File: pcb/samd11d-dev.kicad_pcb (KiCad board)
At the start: 2 copper layers, 30.5 x 29.2 mm, 28 parts, among them J1 Conn_02x05_Odd_Even, J2 USB_B_Micro, J3 Conn_01x08, J4 Conn_01x08, SW1 SW_Push, SW2 SW_Push, U1 ATSAMD11D14A-SS, U3 MCP1700-3302E_SOT23, U4 USBLC6-2SC6, Y1 32.768 kHz

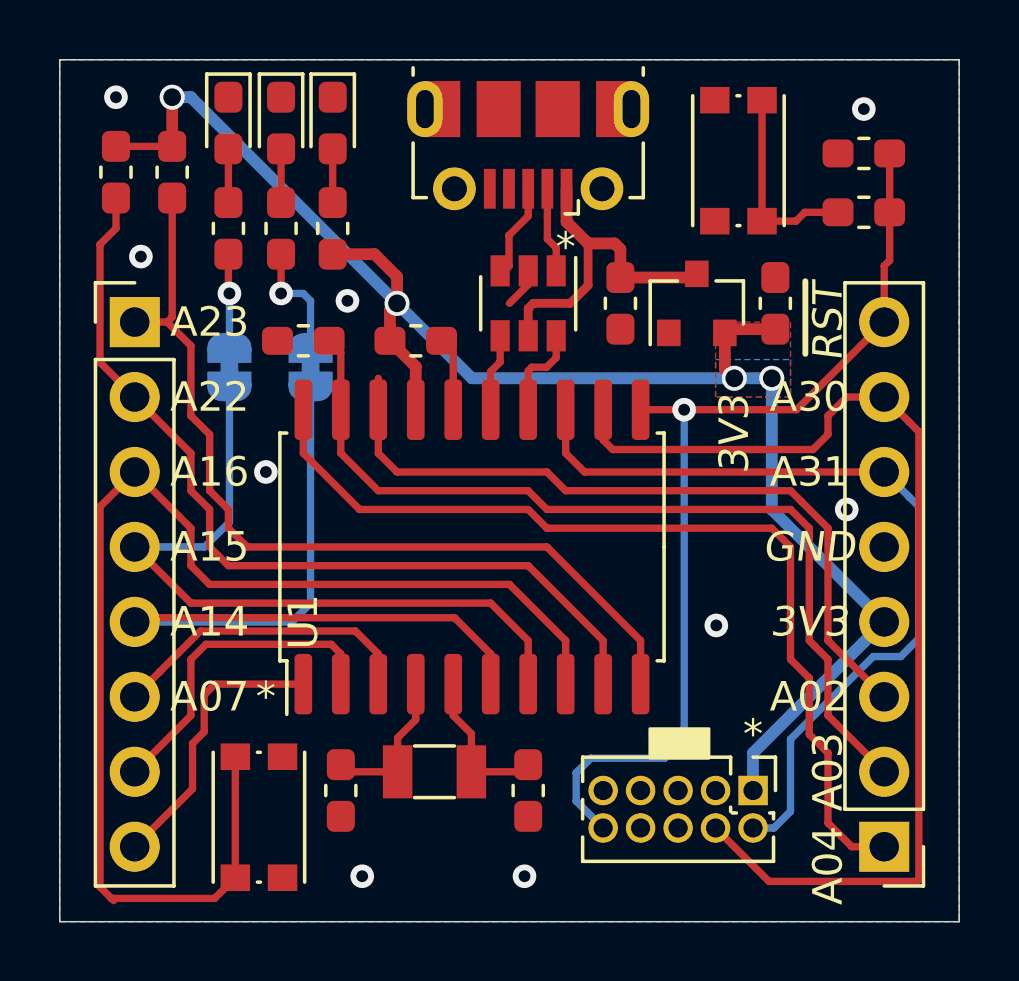
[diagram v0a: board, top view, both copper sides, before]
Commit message: Complete new layout for v0.21
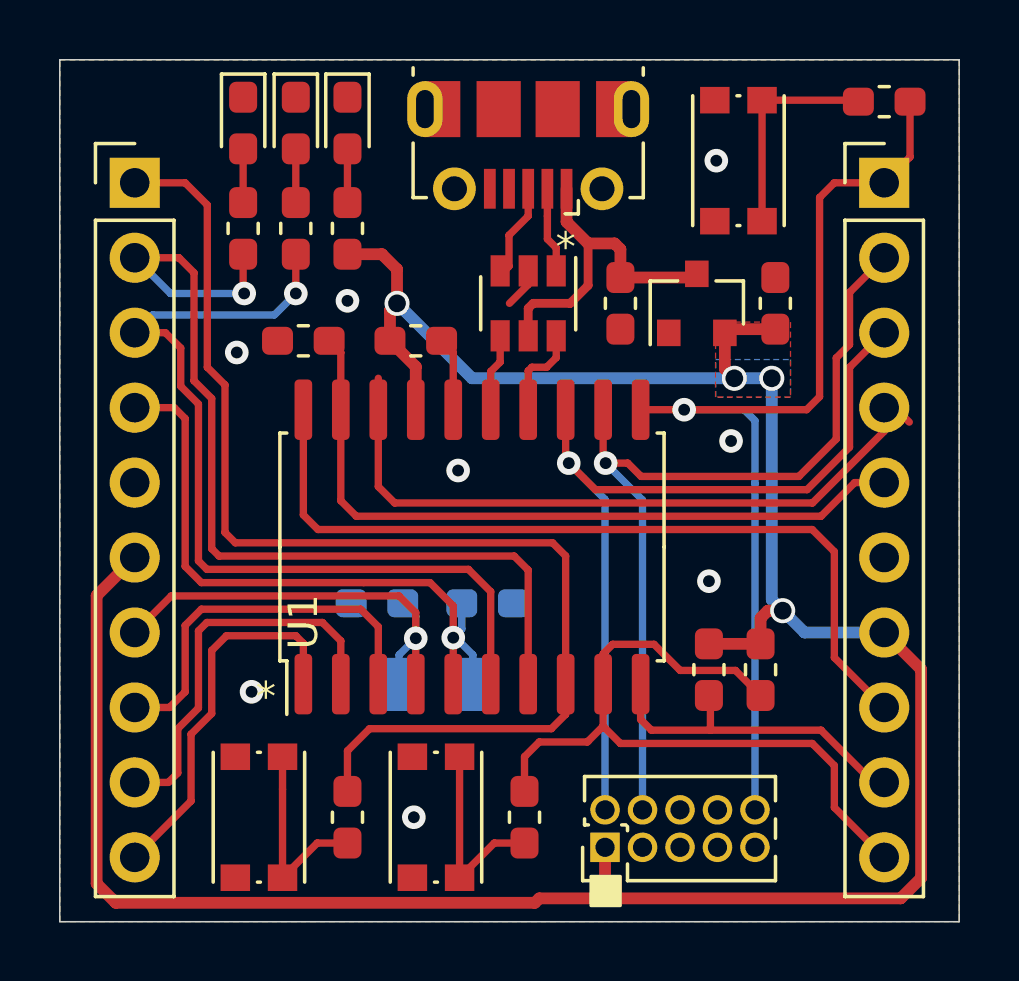
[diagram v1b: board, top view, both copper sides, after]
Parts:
- removed C7: 100n, Capacitor_SMD:C_0603_1608Metric_Pad1.05x0.95mm_HandSolder
- removed JP1, JP2: Jumper_NC_Small, Jumper:SolderJumper-2_P1.3mm_Bridged_RoundedPad1.0x1.5mm
- added R7: 330R, Resistor_SMD:R_0603_1608Metric_Pad1.05x0.95mm_HandSolder, F.Cu at (134.8, 126.5)
- added R8: 330R, Resistor_SMD:R_0603_1608Metric_Pad1.05x0.95mm_HandSolder, F.Cu at (140.8, 126.5)
- added SW3: SW_Push, Button_Switch_SMD:SW_Push_1P1T_NO_CK_KMR2, F.Cu at (137.8, 126.5)
- C1, C2, Y1: moved to B.Cu
- J3, J4: value Conn_01x08 -> Conn_01x10; footprint Connector_PinHeader_2.54mm:PinHeader_1x08_P2.54mm_Vertical -> Connector_PinHeader_2.54mm:PinHeader_1x10_P2.54mm_Vertical
- moved R1 27.6 mm to (148.8, 121.5)
- moved R2 24.8 mm to (147.0, 121.5)
- moved J4 22.5 mm to (152.9, 105.0), turned to 0 degrees
- moved C2 6.49 mm to (139.5, 119.2), turned to 0 degrees
- moved C1 6.46 mm to (135.8, 119.2), turned to 180 degrees
- moved J1 5.37 mm to (143.5, 127.5), turned to 90 degrees
- moved J3 4.72 mm to (127.5, 105.0)
- moved R6 3.81 mm to (152.9, 102.2)
- moved Y1 2.96 mm to (137.8, 122.0)
- moved D1 0.50 mm to (131.2, 103.0)
- moved D2 0.50 mm to (133.0, 103.0)
- moved D3 0.50 mm to (134.8, 103.0)
- moved R3 0.50 mm to (131.2, 106.5)
- moved R4 0.50 mm to (134.8, 106.5)
- moved R5 0.50 mm to (133.0, 106.5)
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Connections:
- C1 pad 1: Net-(C1-Pad1) -> /PA08
- C2 pad 1: Net-(C2-Pad1) -> /PA09
- J3 pad 1: /PA23 -> /PA16
- J3 pad 2: /PA22 -> /PA15
- J3 pad 3: /PA16 -> /PA14
- J3 pad 4: /PA15 -> /PA09
- J3 pad 5: /PA14 -> GND
- J3 pad 6: /PA07 -> +3V3
- J3 pad 7: /PA06 -> /PA08
- J3 pad 8: /PA05 -> /PA07
- J4 pad 1: /PA04 -> /~RST
- J4 pad 2: /PA03 -> /PA30
- J4 pad 3: /PA02 -> /PA31
- J4 pad 4: +3V3 -> /PA02
- J4 pad 5: GND -> /PA03
- J4 pad 6: /PA31 -> GND
- J4 pad 7: /PA30 -> +3V3
- J4 pad 8: /~RST -> /PA04
- R3 pad 1: Net-(JP2-Pad2) -> /PA15
- R5 pad 1: Net-(JP1-Pad2) -> /PA14
- SW2 pad 1: /PA16 -> Net-(R7-Pad1)
- U1 pad 4: Net-(C1-Pad1) -> /PA08
- U1 pad 5: Net-(C2-Pad1) -> /PA09
- Y1 pad 1: Net-(C1-Pad1) -> /PA08
- Y1 pad 2: Net-(C2-Pad1) -> /PA09
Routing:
- net +3V3: track 56.0 -> 90.2 mm
- net /PA09: track 0.00 -> 22.4 mm, vias 0 -> 1
- net /PA23: track 30.2 -> 11.5 mm
- net /PA08: track 0.00 -> 15.9 mm, vias 0 -> 1
- net /PA15: track 24.3 -> 32.3 mm, vias 0 -> 1
- net Net-(R7-Pad1): track 0.00 -> 6.85 mm
- net Net-(R8-Pad1): track 0.00 -> 6.79 mm
- net /PA30: track 36.3 -> 29.7 mm, vias 0 -> 1
- net /PA03: track 30.2 -> 24.7 mm
- net Net-(C2-Pad1): track 5.25 -> 0.00 mm
- net Net-(C1-Pad1): track 5.25 -> 0.00 mm
- net /PA22: track 29.7 -> 25.1 mm
- net Net-(JP1-Pad2): track 4.03 -> 0.00 mm, vias 1 -> 0
- net /PA04: track 31.4 -> 28.1 mm
- net /PA05: track 9.63 -> 12.9 mm
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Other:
- board text added: "A08"
- board text added: "A09"
- board text removed: "SAMD11D-dev v0.2"
- board text removed: "awjlogan 2020"

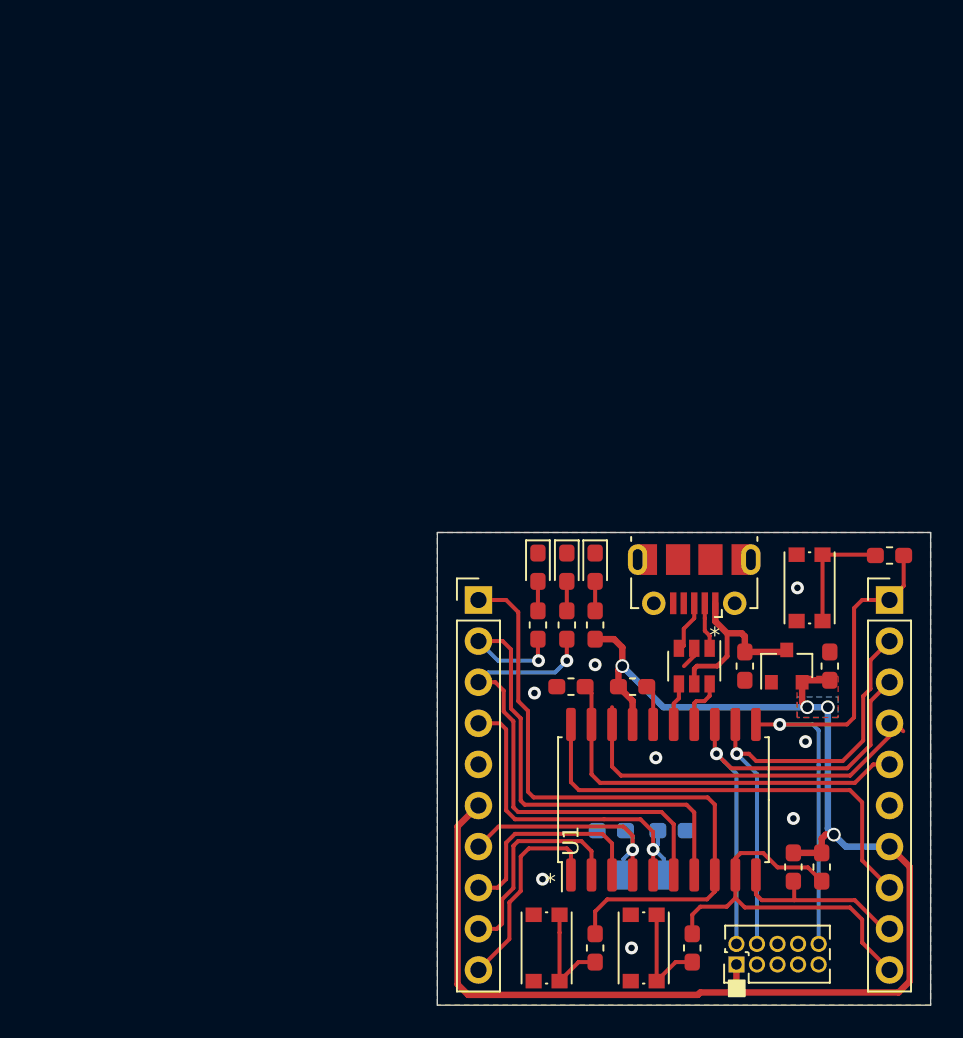
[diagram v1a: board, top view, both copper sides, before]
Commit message: v2.1 manufactured
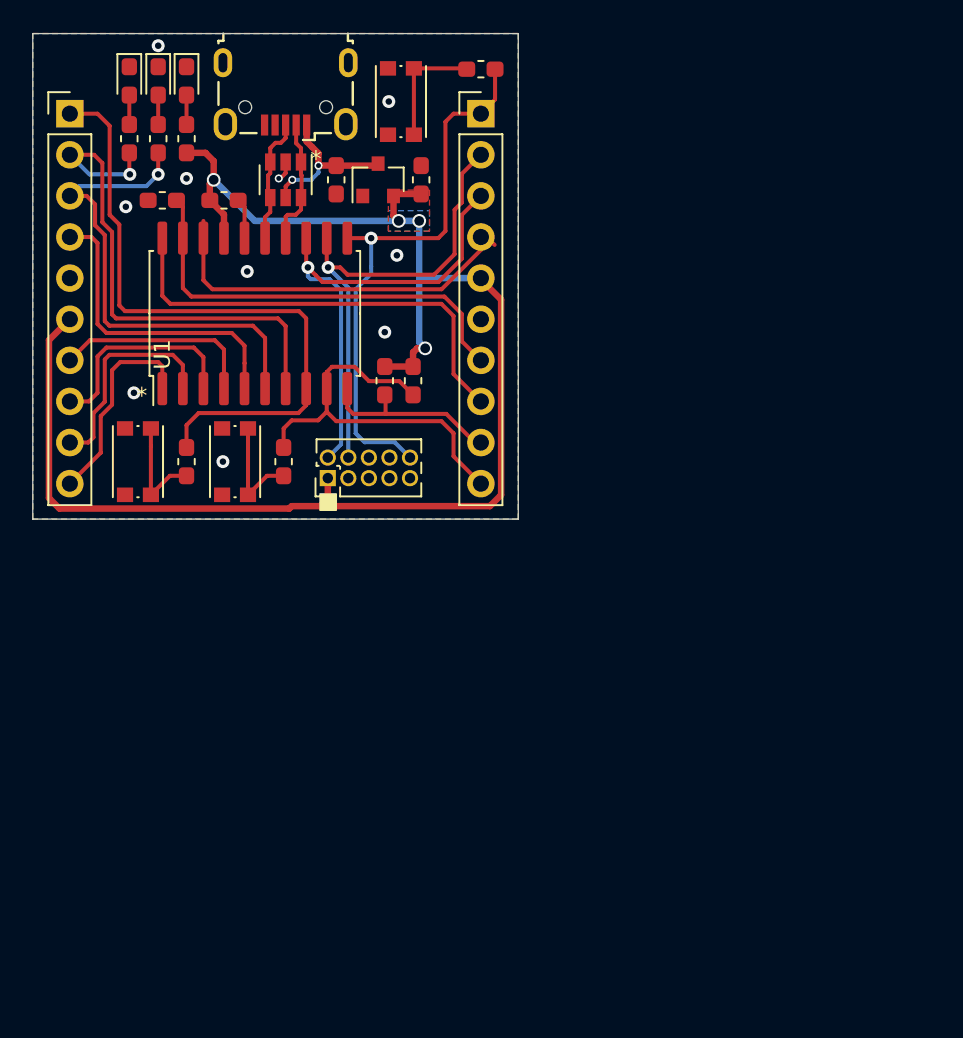
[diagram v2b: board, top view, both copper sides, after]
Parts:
- removed C1, C2: 15p, Capacitor_SMD:C_0603_1608Metric_Pad1.05x0.95mm_HandSolder
- removed Y1: 32.768 kHz, Crystal:Crystal_SMD_3215-2Pin_3.2x1.5mm
- J2: footprint Connector_USB:USB_Micro-B_Molex-105017-0001 -> Connector_USB:USB_Micro-B_Wuerth_629105150521
- moved C3 39.3 mm to (118.8, 79.0)
- moved C4 39.3 mm to (124.0, 79.0)
- moved C5 39.3 mm to (111.8, 80.3)
- moved C6 39.3 mm to (108.0, 80.3)
- moved D1 39.3 mm to (106.0, 72.9)
- moved D2 39.3 mm to (107.8, 72.9)
- moved D3 39.3 mm to (109.5, 72.9)
- moved J3 39.3 mm to (102.3, 75.0)
- moved J4 39.3 mm to (127.7, 75.0)
- moved R1 39.3 mm to (123.5, 91.5)
- moved R2 39.3 mm to (121.8, 91.5)
- moved R3 39.3 mm to (106.0, 76.5)
- moved R4 39.3 mm to (109.5, 76.5)
- moved R5 39.3 mm to (107.8, 76.5)
- moved R6 39.3 mm to (127.7, 72.2)
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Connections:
- J4 pad 5: /PA03 -> +3V3
- J4 pad 7: +3V3 -> /PA03
- U1 pad 14: /USB_ESD_D- -> /USB_D-
- U1 pad 15: /USB_ESD_D+ -> /USB_D+
- U4 pad 4: /USB_ESD_D+ -> /USB_D+
- U4 pad 6: /USB_ESD_D- -> /USB_D-
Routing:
- net +3V3: track 90.2 -> 95.3 mm
- net /USB_D-: track 2.91 -> 7.83 mm
- net /USB_D+: track 3.26 -> 7.97 mm
- net /PA09: track 22.4 -> 19.2 mm, vias 1 -> 0
- net /USB_ESD_D-: track 3.19 -> 0.00 mm
- net /PA08: track 15.9 -> 12.7 mm, vias 1 -> 0
- net /USB_ESD_D+: track 2.64 -> 0.00 mm
- net /PA03: track 24.7 -> 26.8 mm
- net VBUS: track 11.6 -> 10.1 mm, vias 0 -> 2
- net /PA31: track 29.0 -> 30.3 mm
- net /~RST: track 34.3 -> 34.9 mm
- net GND: track 3.86 -> 3.75 mm, vias 8 -> 10
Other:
- board size 30.5 x 29.2 mm -> 30 x 30 mm
- board text added: "SAMD1-DEV AWJL 2020"
